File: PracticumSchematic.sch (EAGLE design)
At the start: 9 parts, among them U1 328P, U2 MMA8452Q, U3 SN74HC595N, U4 SN74HC595N, U5 SN74HC595N, U6 SN74HC595N

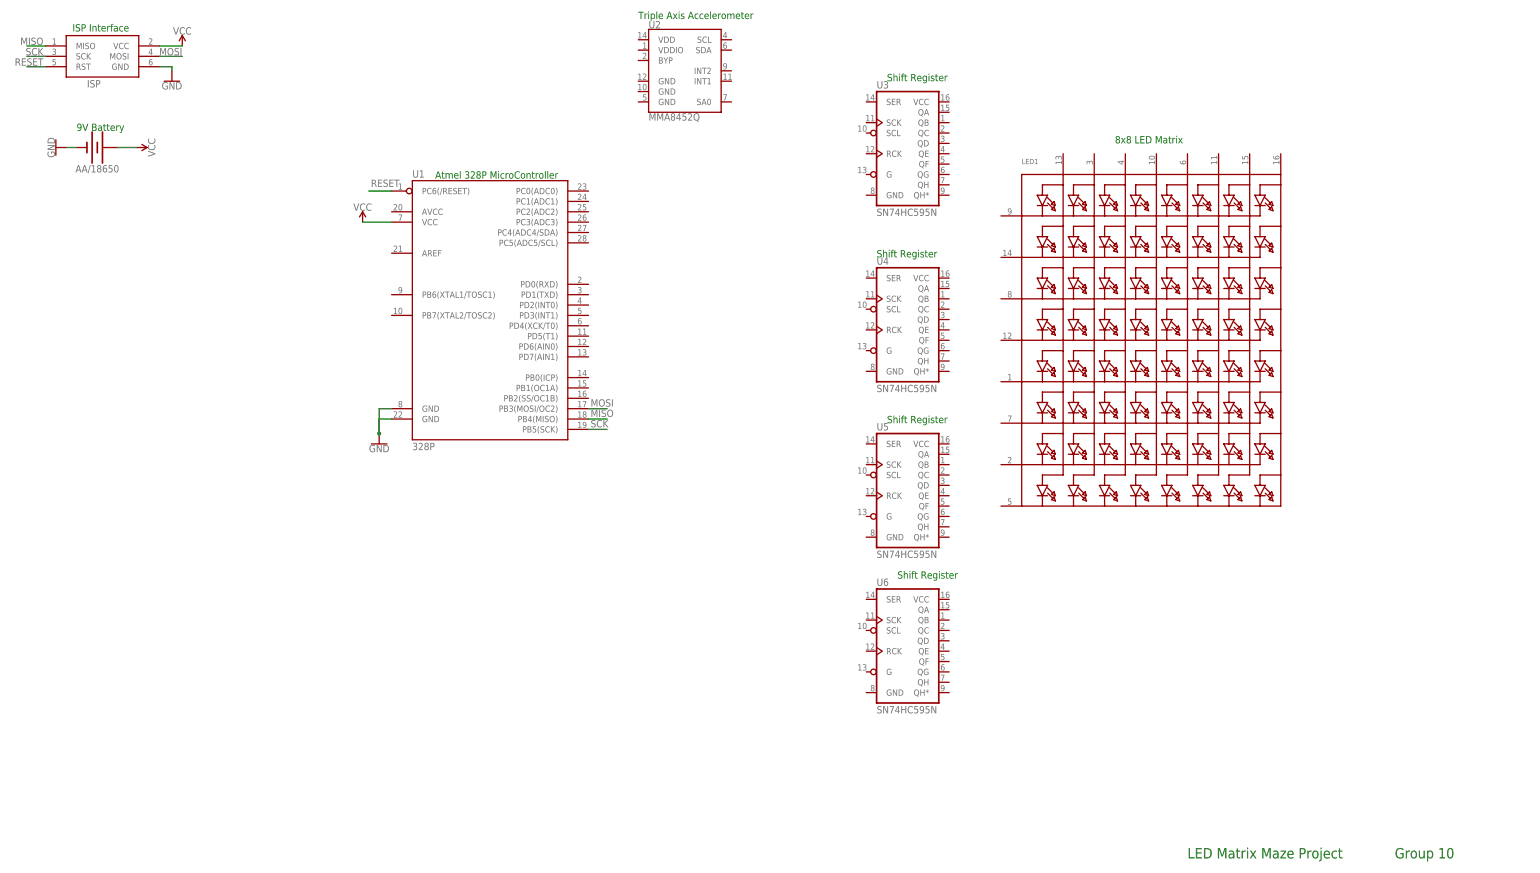
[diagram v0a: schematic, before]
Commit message: Add files via upload
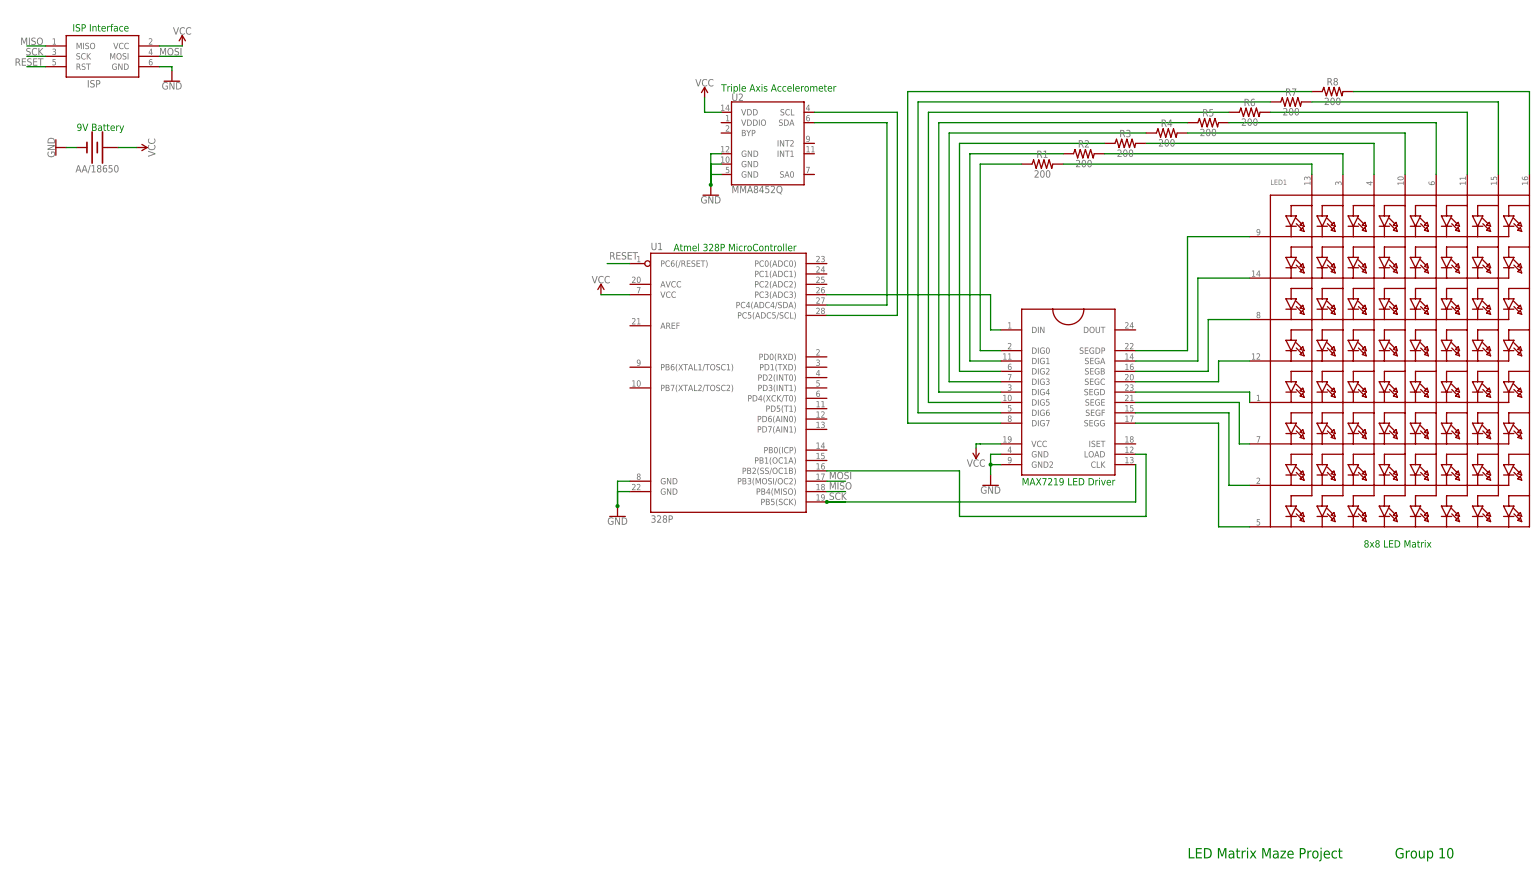
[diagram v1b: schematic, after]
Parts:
- removed U3, U4, U5, U6: SN74HC595N, SparkFun-IC-Logic:74HC595N
- added R1, R2, R3, R4, R5, R6, R7, R8: 200, SparkFun-Resistors:200OHM-0603-1/10W-1%
- added U$1: MAX7219DIP, SparkFun-Retired:MAX7219DIP
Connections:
- new net N$1: LED1.K1, U$1.SEGDP
- new net N$10: R2.1, U$1.DIG1
- new net N$11: R3.1, U$1.DIG2
- new net N$12: R4.1, U$1.DIG3
- new net N$13: R5.1, U$1.DIG4
- new net N$14: R6.1, U$1.DIG5
- new net N$15: R7.1, U$1.DIG6
- new net N$16: R8.1, U$1.DIG7
- new net N$17: U$1.DIN, U1.PC3(ADC3)
- new net N$18: U1.PC5(ADC5/SCL), U2.SCL
- new net N$19: U1.PC4(ADC4/SDA), U2.SDA
- new net N$2: LED1.K2, U$1.SEGA
- new net N$20: U$1.LOAD, U1.PB2(SS/OC1B)
- new net N$21: R1.1, U$1.DIG0
- new net N$22: LED1.A2, R2.2
- new net N$23: LED1.A3, R3.2
- new net N$24: LED1.A4, R4.2
- new net N$25: LED1.A5, R5.2
- new net N$26: LED1.A6, R6.2
- new net N$27: LED1.A7, R7.2
- new net N$28: LED1.A8, R8.2
- new net N$3: LED1.K3, U$1.SEGB
- new net N$4: LED1.K4, U$1.SEGC
- new net N$5: LED1.K5, U$1.SEGD
- new net N$6: LED1.K6, U$1.SEGE
- new net N$7: LED1.K7, U$1.SEGF
- new net N$8: LED1.K8, U$1.SEGG
- new net N$9: LED1.A1, R1.2
- net GND: now also U$1.GND, U$1.GND2, U2.GND@0, U2.GND@1, U2.GND@2
- net SCK: now also U$1.CLK
- net VCC: now also U$1.VCC, U2.VDD
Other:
- note added: "MAX7219 LED Driver"
- note removed: "Shift Register"
- moved on the sheet: LED1, U1, U2
